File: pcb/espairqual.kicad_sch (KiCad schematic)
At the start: 48 parts, among them J1 24VAC, J2 PMSX003, J3 eflashy32, J4 USBC, J5 GCJA5, J6 TEST, J7 AUX, SW1 RESET, U1 BD9G101G, U3 AMS1117-3.3, U4 ESP32-C3-MINI-1

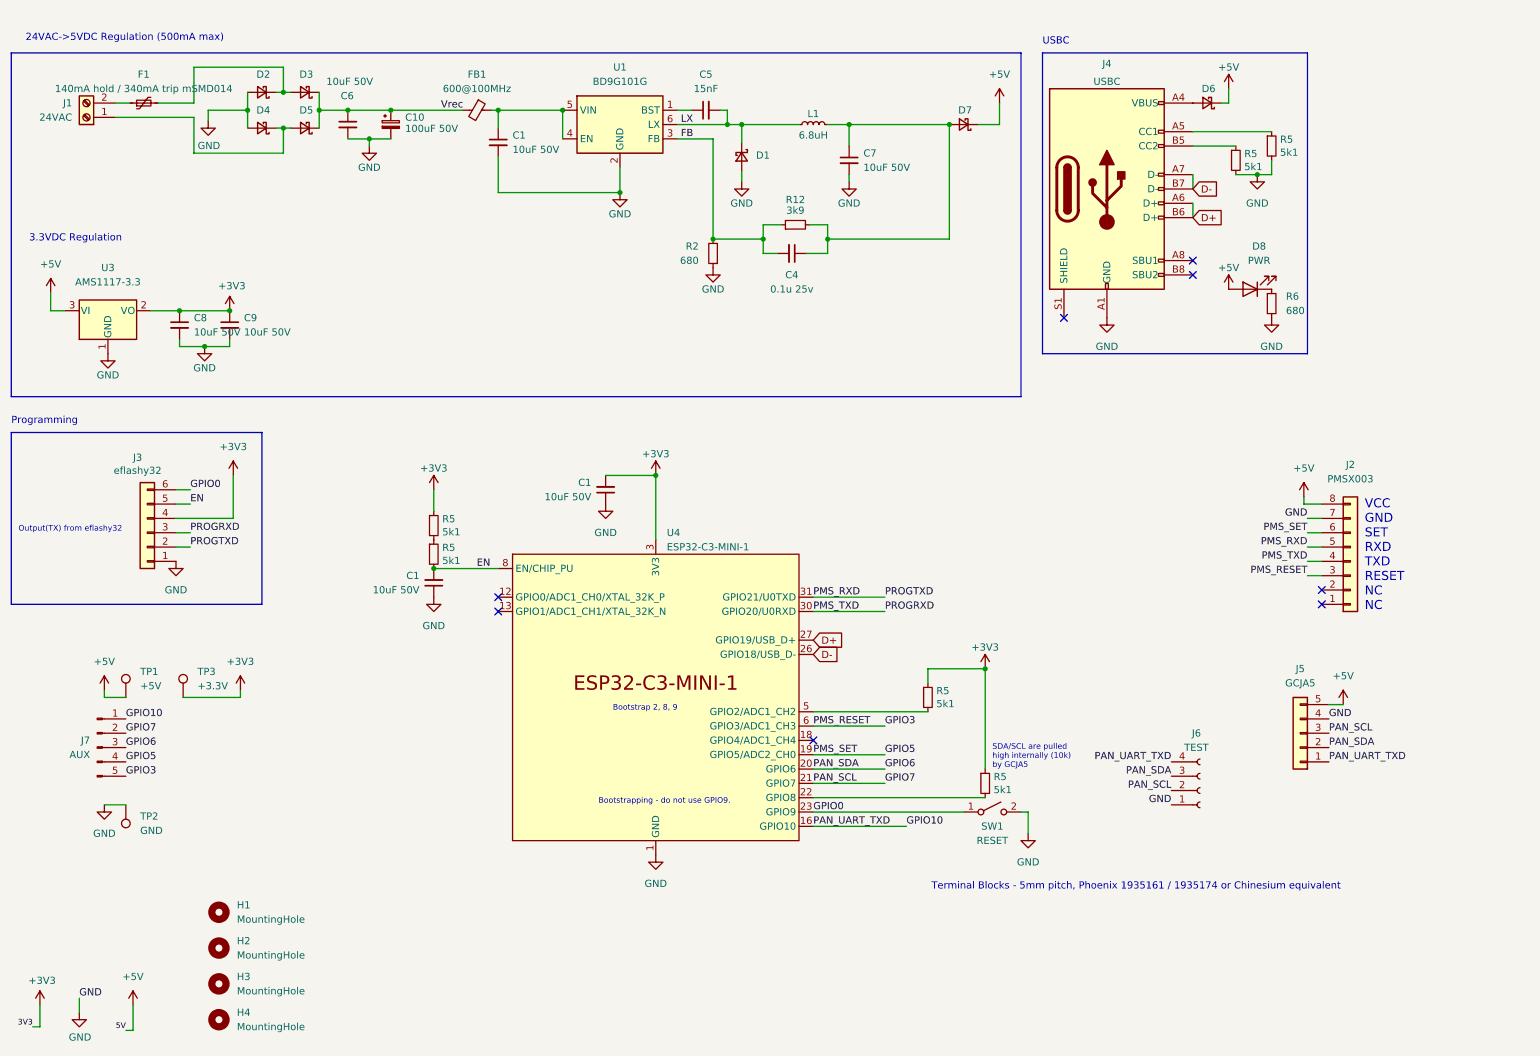
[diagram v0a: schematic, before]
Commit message: touchup before fab
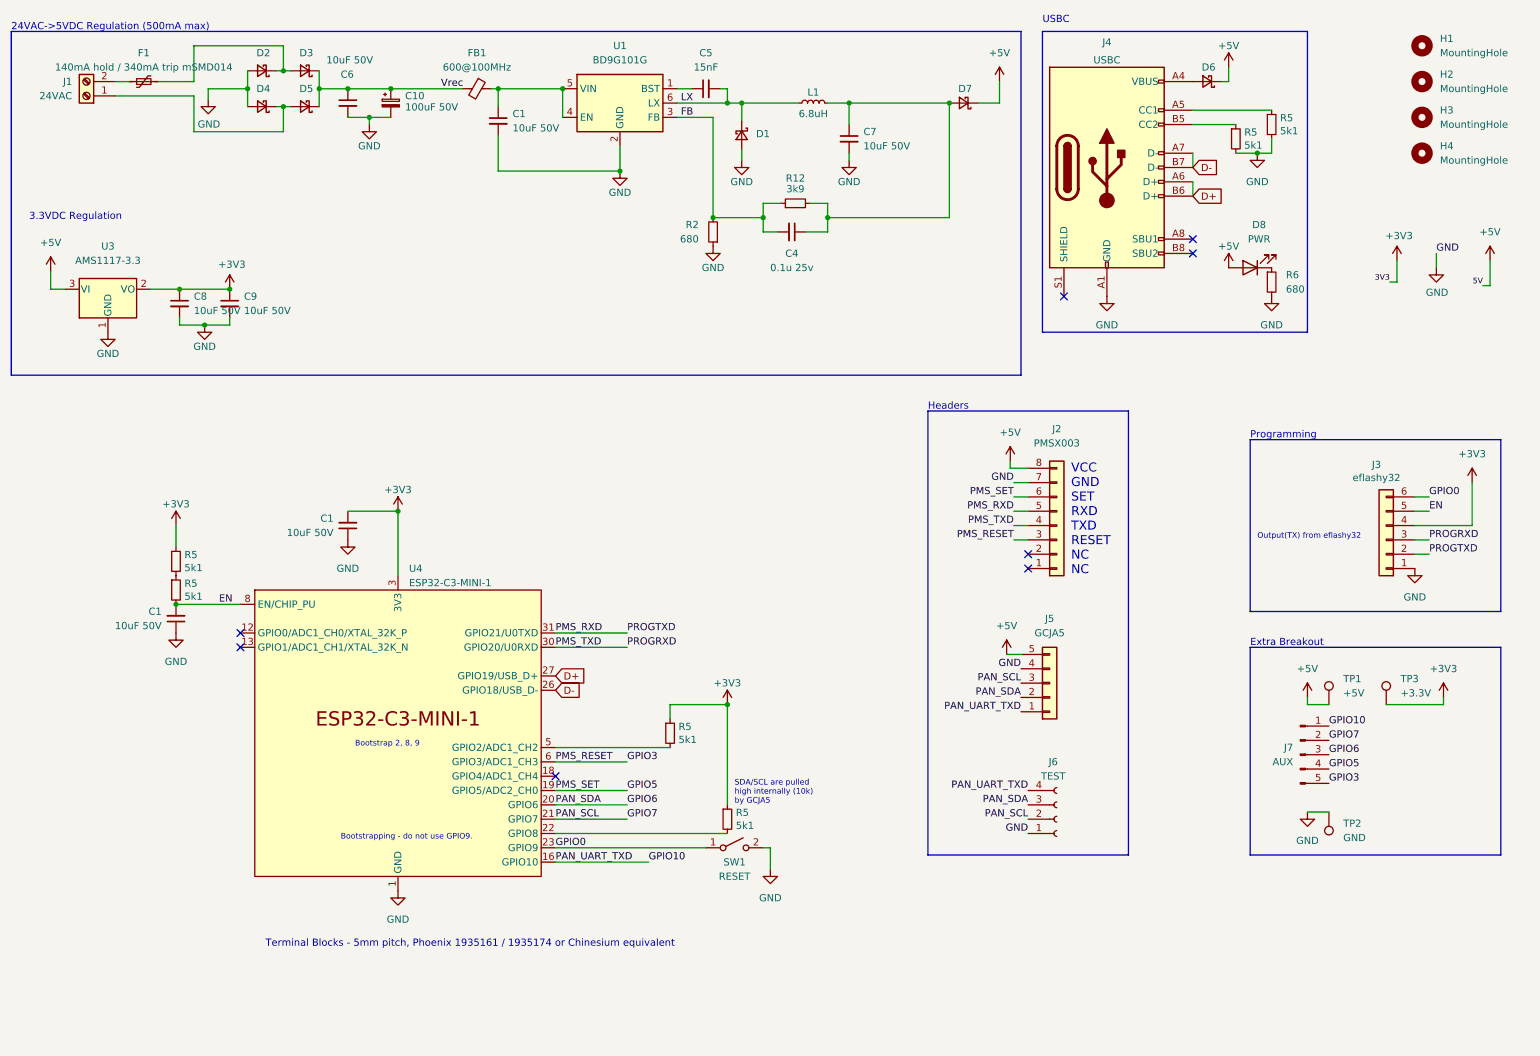
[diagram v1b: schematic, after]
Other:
- note added: "Extra Breakout"
- note added: "Headers"
- moved on the sheet: C1, C10, C4, C5, C6, C7, C8, C9, D1, D2, D3, D4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
